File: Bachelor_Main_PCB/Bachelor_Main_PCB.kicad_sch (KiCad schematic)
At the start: 4 parts

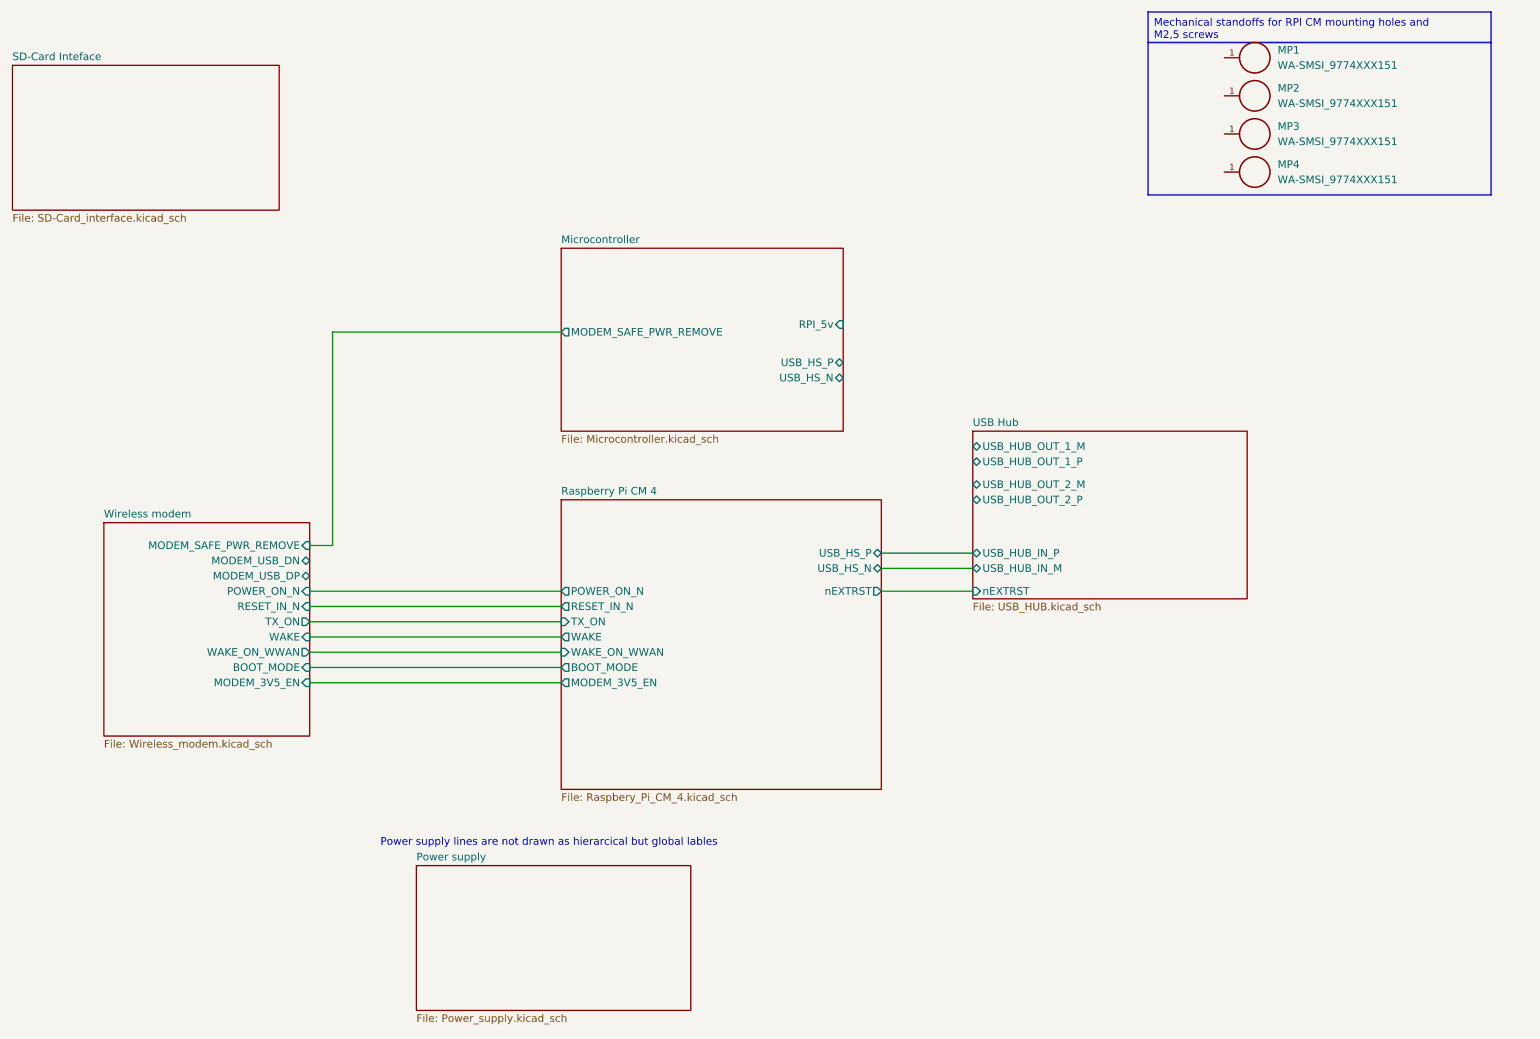
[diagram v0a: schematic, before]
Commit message: Routed Sheeets
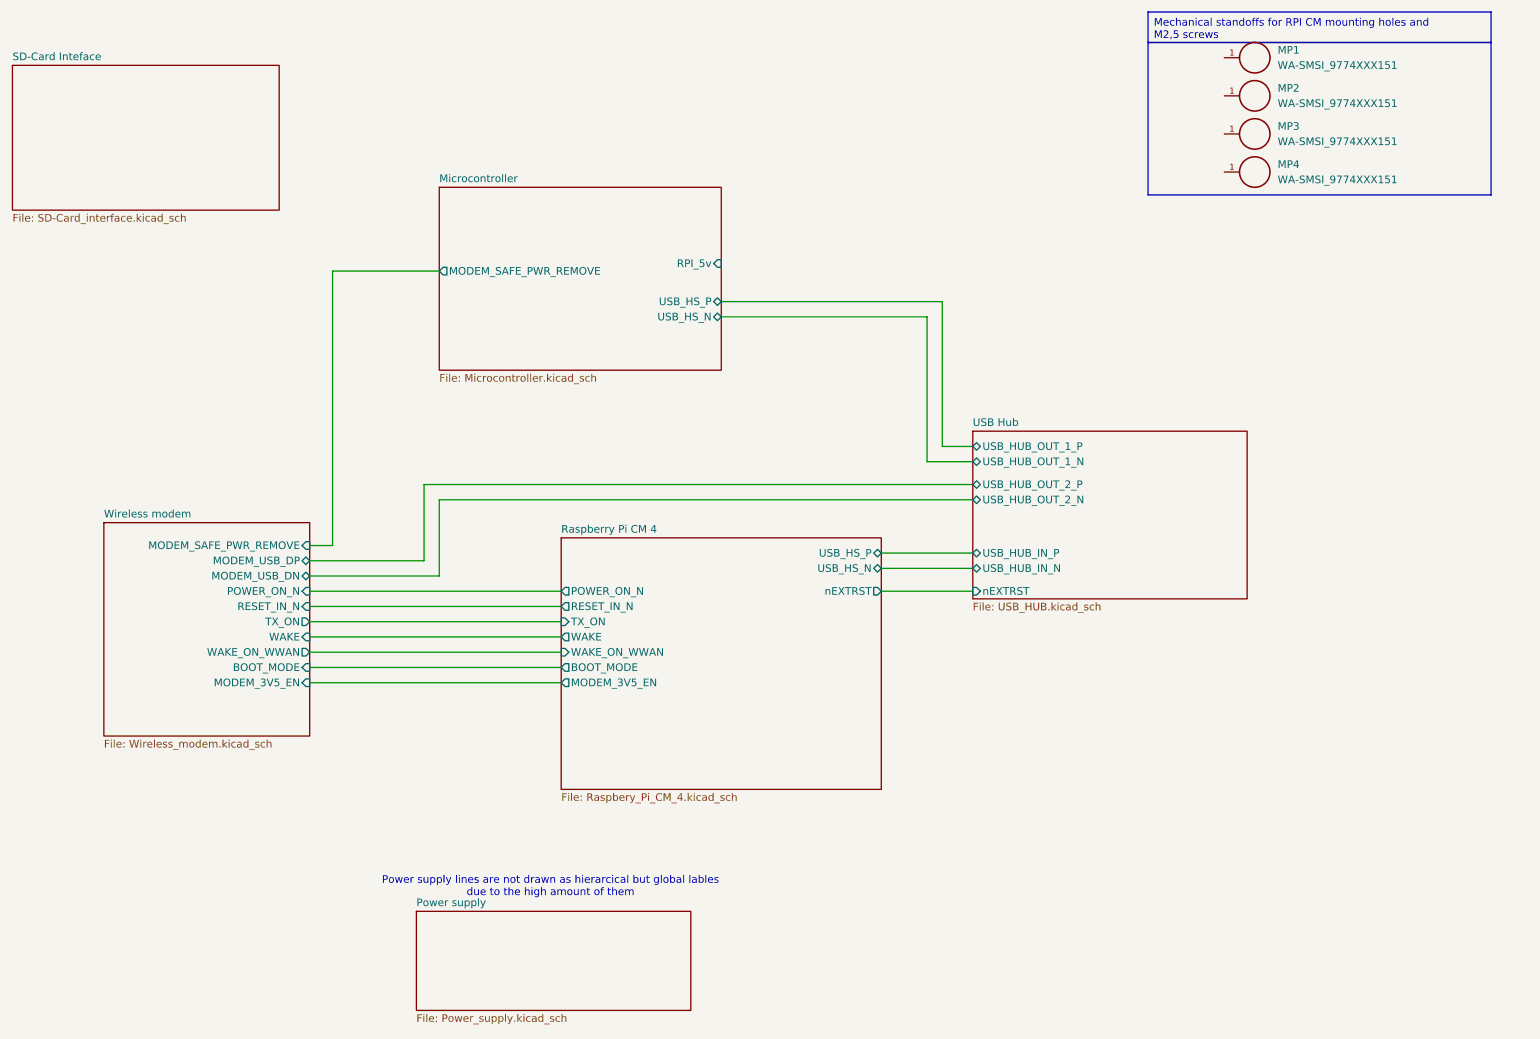
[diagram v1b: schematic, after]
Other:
- sheet USB Hub ports: added USB_HUB_IN_N, USB_HUB_OUT_1_N, USB_HUB_OUT_2_N; removed USB_HUB_IN_M, USB_HUB_OUT_1_M, USB_HUB_OUT_2_M
- note added: "Power supply lines are not drawn as hierarcical but global lables due to the high amount of them"
- note removed: "Power supply lines are not drawn as hierarcical but global lables"
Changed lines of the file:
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@@
 	(generator_version "9.0")
 	(paper "A4")
-	(text "Power supply lines are not drawn as hierarcical but global lables"
+	(text "Power supply lines are not drawn as hierarcical but global lables\ndue to the high amount of them"
 		(exclude_from_sim no)
-		(at 119.888 156.21 0)
+		(at 120.142 163.576 0)
 		(effects
 			(font
@@
 	(wire
 		(pts
+			(xy 80.01 111.76) (xy 101.6 111.76)
+		)
+		(stroke
+			(width 0)
+			(type default)
+		)
+	)
+	(wire
+		(pts
 			(xy 175.26 110.49) (xy 190.5 110.49)
 		)
@@
 	(wire
 		(pts
-			(xy 83.82 71.12) (xy 121.92 71.12)
+			(xy 182.88 92.71) (xy 182.88 68.58)
+		)
+		(stroke
+			(width 0)
+			(type default)
+		)
+	)
+	(wire
+		(pts
+			(xy 99.06 109.22) (xy 80.01 109.22)
+		)
+		(stroke
+			(width 0)
+			(type default)
+		)
+	)
+	(wire
+		(pts
+			(xy 101.6 111.76) (xy 101.6 99.06)
+		)
+		(stroke
+			(width 0)
+			(type default)
+		)
+	)
+	(wire
+		(pts
+			(xy 182.88 68.58) (xy 148.59 68.58)
+		)
+		(stroke
+			(width 0)
+			(type default)
+		)
+	)
+	(wire
+		(pts
+			(xy 83.82 60.96) (xy 101.6 60.96)
+		)
+		(stroke
+			(width 0)
+			(type default)
+		)
+	)
+	(wire
+		(pts
+			(xy 99.06 96.52) (xy 99.06 109.22)
 		)
 		(stroke
@@
 	(wire
 		(pts
+			(xy 190.5 92.71) (xy 182.88 92.71)
+		)
+		(stroke
+			(width 0)
+			(type default)
+		)
+	)
+	(wire
+		(pts
 			(xy 80.01 127) (xy 121.92 127)
 		)
@@
 	(wire
 		(pts
+			(xy 190.5 96.52) (xy 99.06 96.52)
+		)
+		(stroke
+			(width 0)
+			(type default)
+		)
+	)
+	(wire
+		(pts
+			(xy 185.42 90.17) (xy 185.42 66.04)
+		)
+		(stroke
+			(width 0)
+			(type default)
+		)
+	)
+	(wire
+		(pts
 			(xy 80.01 124.46) (xy 121.92 124.46)
 		)
@@
 	(wire
 		(pts
-			(xy 83.82 106.68) (xy 83.82 71.12)
+			(xy 185.42 66.04) (xy 148.59 66.04)
+		)
+		(stroke
+			(width 0)
+			(type default)
+		)
+	)
+	(wire
+		(pts
+			(xy 83.82 106.68) (xy 83.82 60.96)
+		)
+		(stroke
+			(width 0)
+			(type default)
+		)
+	)
+	(wire
+		(pts
+			(xy 101.6 99.06) (xy 190.5 99.06)
 		)
 		(stroke
@@
 		(pts
 			(xy 80.01 119.38) (xy 121.92 119.38)
+		)
+		(stroke
+			(width 0)
+			(type default)
+		)
+	)
+	(wire
+		(pts
+			(xy 190.5 90.17) (xy 185.42 90.17)
 		)
 		(stroke
@@
 		)
 		(pin "MODEM_USB_DN" bidirectional
+			(at 80.01 111.76 0)
+			(effects
+				(font
+					(size 1.27 1.27)
+				)
+				(justify right)
+			)
+		)
+		(pin "MODEM_USB_DP" bidirectional
 			(at 80.01 109.22 0)
-			(effects
-				(font
-					(size 1.27 1.27)
-				)
-				(justify right)
-			)
-		)
-		(pin "MODEM_USB_DP" bidirectional
-			(at 80.01 111.76 0)
 			(effects
 				(font
@@
 	)
 	(sheet
-		(at 121.92 99.06)
-		(size 53.34 48.26)
+		(at 121.92 105.41)
+		(size 53.34 41.91)
 		(exclude_from_sim no)
 		(in_bom yes)
@@
 		)
 		(property "Sheetname" "Raspberry Pi CM 4"
-			(at 121.92 98.3484 0)
+			(at 121.92 104.6984 0)
 			(effects
 				(font
@@
 	)
 	(sheet
-		(at 97.79 160.02)
-		(size 45.72 24.13)
+		(at 97.79 167.64)
+		(size 45.72 16.51)
 		(exclude_from_sim no)
 		(in_bom yes)
@@
 		)
 		(property "Sheetname" "Power supply"
-			(at 97.79 159.3084 0)
+			(at 97.79 166.9284 0)
 			(effects
 				(font
@@
 	)
 	(sheet
-		(at 121.92 57.15)
+		(at 101.6 46.99)
 		(size 46.99 30.48)
 		(exclude_from_sim no)
@@
 		)
 		(property "Sheetname" "Microcontroller"
-			(at 121.92 56.4384 0)
+			(at 101.6 46.2784 0)
 			(effects
 				(font
@@
 		)
 		(property "Sheetfile" "Microcontroller.kicad_sch"
-			(at 121.92 88.2146 0)
+			(at 101.6 78.0546 0)
 			(effects
 				(font
@@
 		)
 		(pin "RPI_5v" input
-			(at 168.91 69.85 0)
+			(at 148.59 59.69 0)
 			(effects
 				(font
@@
 		)
 		(pin "USB_HS_N" bidirectional
-			(at 168.91 78.74 0)
+			(at 148.59 68.58 0)
 			(effects
 				(font
@@
 		)
 		(pin "USB_HS_P" bidirectional
-			(at 168.91 76.2 0)
+			(at 148.59 66.04 0)
 			(effects
 				(font
@@
 		)
 		(pin "MODEM_SAFE_PWR_REMOVE" output
-			(at 121.92 71.12 180)
+			(at 101.6 60.96 180)
 			(effects
 				(font
@@
 			)
 		)
-		(pin "USB_HUB_IN_M" bidirectional
-			(at 190.5 110.49 180)
-			(effects
-				(font
-					(size 1.27 1.27)
-				)
-				(justify left)
-			)
-		)
 		(pin "USB_HUB_IN_P" bidirectional
 			(at 190.5 107.95 180)
@@
 			)
 		)
-		(pin "USB_HUB_OUT_1_M" bidirectional
+		(pin "USB_HUB_OUT_1_P" bidirectional
 			(at 190.5 90.17 180)
 			(effects
@@
 			)
 		)
-		(pin "USB_HUB_OUT_1_P" bidirectional
+		(pin "USB_HUB_OUT_2_P" bidirectional
+			(at 190.5 96.52 180)
+			(effects
+				(font
+					(size 1.27 1.27)
+				)
+				(justify left)
+			)
+		)
+		(pin "USB_HUB_IN_N" bidirectional
+			(at 190.5 110.49 180)
+			(effects
+				(font
+					(size 1.27 1.27)
+				)
+				(justify left)
+			)
+		)
+		(pin "USB_HUB_OUT_1_N" bidirectional
 			(at 190.5 92.71 180)
 			(effects
@@
 			)
 		)
-		(pin "USB_HUB_OUT_2_M" bidirectional
-			(at 190.5 96.52 180)
-			(effects
-				(font
-					(size 1.27 1.27)
-				)
-				(justify left)
-			)
-		)
-		(pin "USB_HUB_OUT_2_P" bidirectional
+		(pin "USB_HUB_OUT_2_N" bidirectional
 			(at 190.5 99.06 180)
 			(effects
